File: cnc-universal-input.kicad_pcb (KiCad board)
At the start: 2 copper layers, 96.5 x 96.5 mm, 161 parts, among them J1 SA, J10 pwr-in, J11 output, J12 USB_B_Mini, J13 ext-pwr, J2 SB, J3 SC, J4 SD, J5 SE, J6 SF, J7 SG, J8 SH, J9 AVR-ISP-6, Q1 2N7002, Q10 IRLML2244TRPBF, Q11 2N7002, Q12 2N7002, Q13 2N7002, Q2 2N7002, Q3 2N7002, Q4 2N7002, Q5 2N7002, Q6 2N7002, Q7 2N7002, Q8 2N7002, Q9 2N7002, SW1 RESET, SW2 BTN, U1 ATmega328PB, U10 SFH617A-4, U11 SFH617A-4, U12 SFH617A-4, U13 SFH617A-4, U14 SFH617A-4, U15 SFH617A-4, U16 SFH617A-4, U17 SFH617A-4, U18 CH340G, U2 74HC595, U3 74HC595, U4 74HC595, U5 4051, U6 L7812, U7 L7805, U8 LM7321, U9 SFH617A-4, Y1 20Mhz, Y2 12MHz

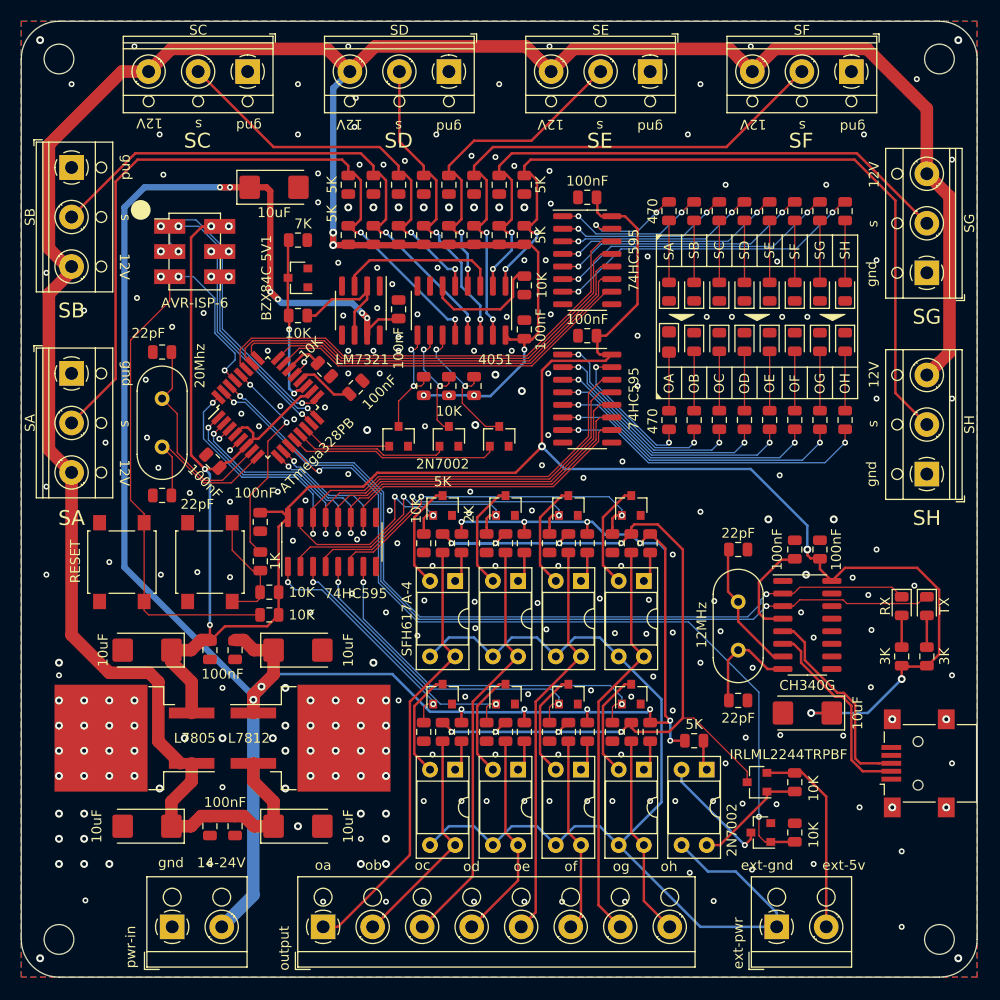
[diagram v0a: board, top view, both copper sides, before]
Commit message: Cleanup
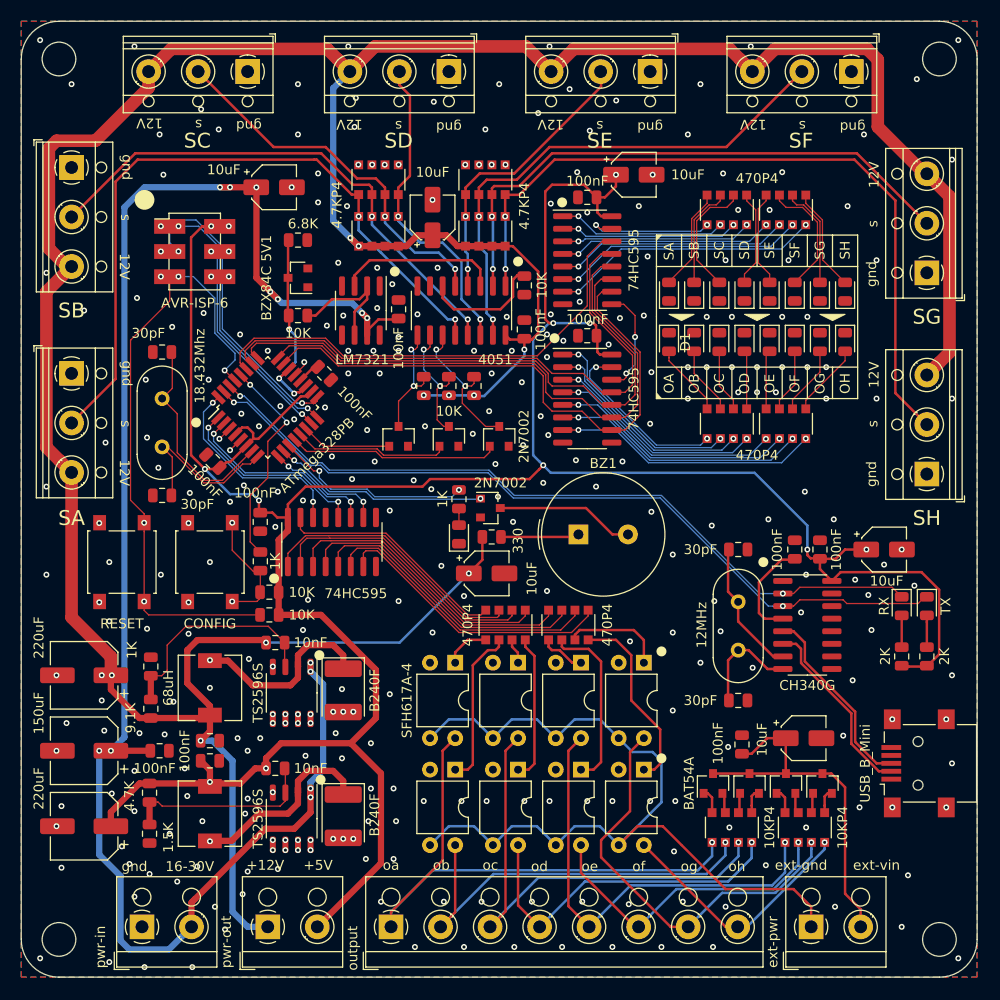
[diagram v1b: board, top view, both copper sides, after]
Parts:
- removed Q10: IRLML2244TRPBF, Package_TO_SOT_SMD:SOT-23
- removed Q2, Q3, Q4, Q5, Q6, Q7, Q8, Q9: 2N7002, Package_TO_SOT_SMD:SOT-23
- removed R10, R11, R12, R13, R14, R15, R16, R2, R3, R4, R44, R45, R46, R47, R5, R56, R57, R58, R59, R6, R7, R8, R9: 5K, Resistor_SMD:R_0805_2012Metric
- removed R18, R19, R20, R21, R22, R23, R24, R25, R26, R27, R28, R29, R30, R31, R32, R33: 470, Resistor_SMD:R_0805_2012Metric
- removed R36, R37, R38, R39, R48, R49, R50, R51: 2K, Resistor_SMD:R_0805_2012Metric
- removed R40, R41, R42, R43, R52, R53, R54, R55, R61, R62, R63: 10K, Resistor_SMD:R_0805_2012Metric
- removed U17: SFH617A-4, Package_DIP:DIP-4_W7.62mm_Socket
- removed U7: L7805, Package_TO_SOT_SMD:TO-263-2
- added BZ1: Buzzer, Buzzer_Beeper:Buzzer_TDK_PS1240P02BT_D12.2mm_H6.5mm, F.Cu at (231.5, -57.4)
- added C24: 10nF, Capacitor_SMD:C_0805_2012Metric, F.Cu at (200.9, -46.5)
- added C25: 10uF, Capacitor_SMD:CP_Elec_4x5.4, F.Cu at (254.3, -36.8)
- added C26: 100nF, Capacitor_SMD:C_0805_2012Metric, F.Cu at (248.0, -36.2)
- added C27: 10uF, Capacitor_SMD:CP_Elec_4x5.4, F.Cu at (216.8, -89.4)
- added C28: 10uF, Capacitor_SMD:CP_Elec_4x5.4, F.Cu at (222.2, -53.5)
- added D20: B240F, Diode_SMD:D_2114_3652Metric, F.Cu at (207.8, -29.0)
- added D21: B240F, Diode_SMD:D_2114_3652Metric, F.Cu at (207.8, -41.7)
- added D22: LEDB, Diode_SMD:D_0805_2012Metric, F.Cu at (219.5, -57.4)
- added D23: BAT54A, Package_TO_SOT_SMD:SOT-23, F.Cu at (245.1, -32.3)
- added D24: BAT54A, Package_TO_SOT_SMD:SOT-23, F.Cu at (248.8, -32.3)
- added D25: BAT54A, Package_TO_SOT_SMD:SOT-23, F.Cu at (256.2, -32.3)
- added D26: BAT54A, Package_TO_SOT_SMD:SOT-23, F.Cu at (252.5, -32.3)
- added J14: 2PT, TerminalBlock_RND:TerminalBlock_RND_205-00001_1x02_P5.00mm_Horizontal, F.Cu at (200.2, -17.8)
- added L1: 68uH, Inductor_SMD:L_6.3x6.3_H3, F.Cu at (194.3, -29.2)
- added L2: 68uH, Inductor_SMD:L_6.3x6.3_H3, F.Cu at (194.3, -41.9)
- added R72: 4.7K, Resistor_SMD:R_0805_2012Metric, F.Cu at (188.2, -31.3)
- added R73: 1.5K, Resistor_SMD:R_0805_2012Metric, F.Cu at (188.2, -27.2)
- added R74: 9.1K, Resistor_SMD:R_0805_2012Metric, F.Cu at (188.3, -39.8)
- added R75: 1K, Resistor_SMD:R_0805_2012Metric, F.Cu at (188.3, -44.1)
- added RN1: 10KP4, Resistor_SMD:R_Array_Convex_4x1206, F.Cu at (247.0, -27.8)
- added RN10: 4.7KP4, Resistor_SMD:R_Array_Convex_4x1206, F.Cu at (222.1, -93.2)
- added RN11: 470P4, Resistor_SMD:R_Array_Convex_4x1206, F.Cu at (224.2, -48.3)
- added RN12: 470P4, Resistor_SMD:R_Array_Convex_4x1206, F.Cu at (230.5, -48.3)
- added RN2: 10KP4, Resistor_SMD:R_Array_Convex_4x1206, F.Cu at (254.4, -27.8)
- added RN3: 470P4, Resistor_SMD:R_Array_Convex_4x1206, F.Cu at (246.5, -90.2)
- added RN4: 470P4, Resistor_SMD:R_Array_Convex_4x1206, F.Cu at (252.5, -90.2)
- added RN5: 470P4, Resistor_SMD:R_Array_Convex_4x1206, F.Cu at (246.5, -68.6)
- added RN6: 470P4, Resistor_SMD:R_Array_Convex_4x1206, F.Cu at (252.5, -68.6)
- added RN7: 4.7KP4, Resistor_SMD:R_Array_Convex_4x1206, F.Cu at (211.3, -88.0)
- added RN8: 4.7KP4, Resistor_SMD:R_Array_Convex_4x1206, F.Cu at (211.3, -93.2)
- added RN9: 4.7KP4, Resistor_SMD:R_Array_Convex_4x1206, F.Cu at (222.1, -88.0)
- added U19: TS2596S, Package_SO:SOP-8_3.9x4.9mm_P1.27mm, F.Cu at (202.6, -28.7)
- C1, C11, C12, C2: value 22pF -> 30pF
- C10, C22: footprint Capacitor_Tantalum_SMD:CP_EIA-6032-28_Kemet-C -> Capacitor_SMD:CP_Elec_4x5.4
- C14, C8: value 10uF -> 100nF; footprint Capacitor_Tantalum_SMD:CP_EIA-6032-28_Kemet-C -> Capacitor_SMD:C_0805_2012Metric
- C15: value 100nF -> 10nF
- C3: value 10uF -> 150uF; footprint Capacitor_Tantalum_SMD:CP_EIA-6032-28_Kemet-C -> Capacitor_SMD:CP_Elec_6.3x7.7
- C5: value 100nF -> 10uF; footprint Capacitor_SMD:C_0805_2012Metric -> Capacitor_SMD:CP_Elec_4x5.4
- C6: value 100nF -> 220uF; footprint Capacitor_SMD:C_0805_2012Metric -> Capacitor_SMD:CP_Elec_6.3x7.7
- C7: value 10uF -> 220uF; footprint Capacitor_Tantalum_SMD:CP_EIA-6032-28_Kemet-C -> Capacitor_SMD:CP_Elec_6.3x7.7
- D1: value OA -> LEDO; footprint Diode_SMD:D_0805_2012Metric_Pad1.15x1.40mm_HandSolder -> LED_SMD:LED_0805_2012Metric
- D10: value SB -> LEDB
- D11: value SC -> LEDB
- D12: value SD -> LEDB
- D13: value SE -> LEDB
- D14: value SF -> LEDB
- D15: value SG -> LEDB
- D16: value SH -> LEDB
- D18: value RX -> LEDB
- D19: value TX -> LEDO
- D2: value OB -> LEDO
- D3: value OC -> LEDO
- D4: value OD -> LEDO
- D5: value OE -> LEDO
- D6: value OF -> LEDO
- D7: value OG -> LEDO
- D8: value OH -> LEDO
- D9: value SA -> LEDB
- J1: value SA -> 3PT
- J10: value pwr-in -> 2PT
- J11: value output -> 8PT
- J13: value ext-pwr -> 2PT
- J2: value SB -> 3PT
- J3: value SC -> 3PT
- J4: value SD -> 3PT
- J5: value SE -> 3PT
- J6: value SF -> 3PT
- J7: value SG -> 3PT
- J8: value SH -> 3PT
- R1: value 5K -> 330
- R35: value 7K -> 6.8K
- R60: value 5K -> 1K
- R66, R67: value 3K -> 2K
- U10, U11, U12, U13, U14, U15, U16, U9: footprint Package_DIP:DIP-4_W7.62mm_Socket -> Package_DIP:DIP-4_W7.62mm
- U6: value L7812 -> TS2596S; footprint Package_TO_SOT_SMD:TO-263-2 -> Package_SO:SOP-8_3.9x4.9mm_P1.27mm
- Y1: value 20Mhz -> 18.432Mhz
- moved C5 77.1 mm to (237.1, -93.7), turned to 0 degrees
- moved R60 34.0 mm to (219.5, -61.0), turned to 270 degrees
- moved R1 33.7 mm to (222.8, -57.1), turned to 0 degrees
- moved C7 26.4 mm to (181.6, -43.2), turned to 180 degrees
- moved C3 23.9 mm to (181.6, -35.6), turned to 180 degrees
- moved C6 21.8 mm to (181.6, -27.9), turned to 180 degrees
- moved C10 18.2 mm to (262.4, -55.9), turned to 0 degrees
- moved C8 12.9 mm to (194.3, -34.5), turned to 0 degrees
- moved C4 12.7 mm to (189.2, -35.6), turned to 0 degrees
- moved C14 10.7 mm to (194.3, -36.6), turned to 0 degrees
- moved C15 8.82 mm to (200.9, -33.8), turned to 0 degrees
- moved U11 8.25 mm to (225.4, -44.5)
- moved U13 8.25 mm to (231.8, -44.5)
- moved U15 8.25 mm to (238.1, -44.5)
- moved U9 8.25 mm to (219.1, -44.5)
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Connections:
- net /IN-SER renamed /DISP-SER
- net /OA renamed /BA
- net /OB renamed /BB
- net /OC renamed /BC
- net /OD renamed /BD
- net /OE renamed /BE
- net /OF renamed /BF
- net /OG renamed /BG
- net /OH renamed /BH
- C15 pad 1: +12V -> +5V
- C15 pad 2: GND -> Net-(C15-Pad2)
- C5 pad 1: +12V -> +5V
- Q1 pad 1: /OUT-A -> /TO
- Q1 pad 3: Net-(Q1-Pad3) -> Net-(BZ1-Pad2)
- R1 pad 2: /SA -> Net-(BZ1-Pad1)
- R60 pad 1: +24V -> Net-(R60-Pad1)
- U1 pad 1: /~OUT-OE -> /OUT-RCLK
- U1 pad 10: /~OUT-SRCLR -> /TO
- U1 pad 11: /EN-PULLUP -> Net-(R60-Pad1)
- U1 pad 2: /OUT-RCLK -> /OUT-SRCLK
- U1 pad 22: Net-(R63-Pad2) -> /ASIN
- U1 pad 23: /~IN-SRCLR -> /~DISP-SRCLR
- U1 pad 24: /IN-SRCLK -> /DISP-SRCLK
- U1 pad 25: /IN-RCLK -> /DISP-RCLK
- U1 pad 26: /~IN-OE -> /~DISP-OE
- U1 pad 9: /OUT-SRCLK -> /~OUT-SRCLR
- U10 pad 1: Net-(R37-Pad2) -> /POB
- U10 pad 2: Net-(Q2-Pad3) -> GND
- U11 pad 1: Net-(R38-Pad2) -> /POC
- U11 pad 2: Net-(Q3-Pad3) -> GND
- U12 pad 1: Net-(R39-Pad2) -> /POD
- U12 pad 2: Net-(Q4-Pad3) -> GND
- U13 pad 1: Net-(R48-Pad2) -> /POE
- U13 pad 2: Net-(Q5-Pad3) -> GND
- U14 pad 1: Net-(R49-Pad2) -> /POF
- U14 pad 2: Net-(Q6-Pad3) -> GND
- U15 pad 1: Net-(R50-Pad2) -> /POG
- U15 pad 2: Net-(Q7-Pad3) -> GND
- U16 pad 1: Net-(R51-Pad2) -> /POH
- U16 pad 2: Net-(Q8-Pad3) -> GND
- U2 pad 10: /~OUT-SRCLR -> /~DISP-SRCLR
- U2 pad 11: /OUT-SRCLK -> /DISP-SRCLK
- U2 pad 12: /OUT-RCLK -> /DISP-RCLK
- U2 pad 13: /~OUT-OE -> /~DISP-OE
- U2 pad 14: /OUT-SER -> /DISP-SER2
- U3 pad 13: /~OUT-OE -> GND
- U4 pad 10: /~IN-SRCLR -> /~DISP-SRCLR
- U4 pad 11: /IN-SRCLK -> /DISP-SRCLK
- U4 pad 12: /IN-RCLK -> /DISP-RCLK
- U4 pad 13: /~IN-OE -> /~DISP-OE
- U4 pad 9: (no net) -> /DISP-SER2
- U6 pad 2: GND -> Net-(D21-Pad1)
- U6 pad 3: +12V -> Net-(C24-Pad2)
- U9 pad 1: Net-(R36-Pad2) -> /POA
- U9 pad 2: Net-(Q1-Pad3) -> GND
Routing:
- net /BIAS: track 90.1 -> 0.00 mm, vias 8 -> 0
- net /EN-PULLUP: track 81.6 -> 0.00 mm, vias 2 -> 0
- net +24V: track 236.8 -> 170.1 mm, vias 18 -> 13
- net /~DISP-OE: track 0.00 -> 60.1 mm
- net /DISP-RCLK: track 0.00 -> 59.9 mm
- net /~OUT-OE: track 58.8 -> 0.00 mm, vias 2 -> 0
- net /~DISP-SRCLR: track 0.00 -> 58.3 mm
- net /DISP-SRCLK: track 0.00 -> 57.3 mm
- net +5V: track 235.6 -> 284.0 mm, vias 8 -> 12
- net /~IN-OE: track 46.2 -> 0.00 mm
- net +12V: track 294.4 -> 339.5 mm, vias 6 -> 11
- net /IN-RCLK: track 44.0 -> 0.00 mm
- net /OUT-SER: track 62.9 -> 20.8 mm
- net /IN-SRCLK: track 39.3 -> 0.00 mm
- net /OUT-RCLK: track 57.7 -> 20.0 mm
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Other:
- outline, holes or cut-outs redrawn
- board text added: "+12V"
- board text added: "+5V"
- board text added: "16-30V"
- board text added: "3.4mm"
- board text added: "88.9"
- board text added: "BAUD 115200"
- board text added: "CONFIG"
- board text added: "OA"
- board text added: "OB"
- board text added: "OC"
- board text added: "OD"
- board text added: "OE"
- board text added: "OF"
- board text added: "OG"
- board text added: "OH"
- board text added: "RX"
- board text added: "TX"
- board text added: "UCNC"
- board text added: "ext-pwr"
- board text added: "ext-vin"
- board text added: "output"
- board text added: "pwr-in"
- board text added: "pwr-out"
- board text added: "v1.3"
- board text removed: "14-24V"
- board text removed: "ext-5v"
- board text removed: "v1.0"
